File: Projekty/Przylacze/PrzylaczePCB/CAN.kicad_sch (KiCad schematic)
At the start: 49 parts, among them SW1 SW_SPDT, SW2 SW_SPDT, SW3 SW_SPDT, SW4 SW_SPDT, SW5 SW_SPDT, SW6 SW_SPDT, SW7 SW_SPDT, SW8 SW_SPDT, U1 MCP2515-xSO, U2 TJA1055T_3_C,518, U3 MCP2561-E-P, Y1 20MHz

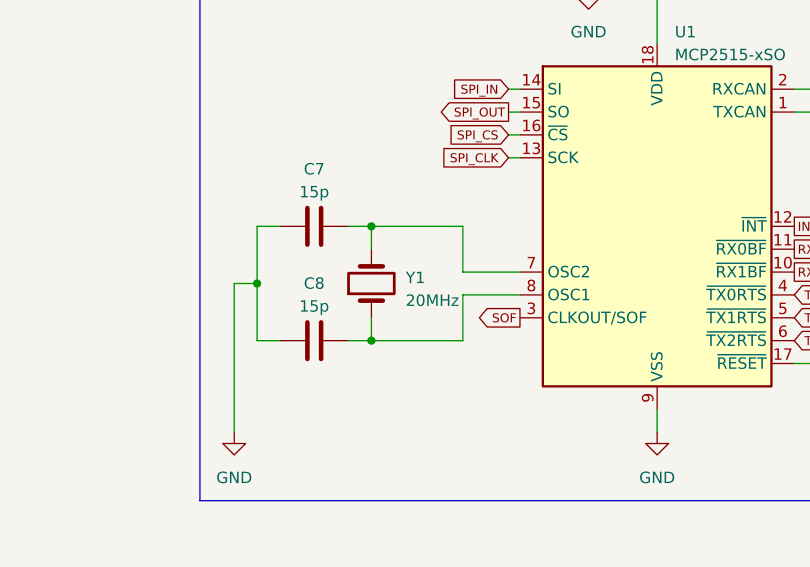
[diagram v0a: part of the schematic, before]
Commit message: Przyłącze - projekt PCB v0.2
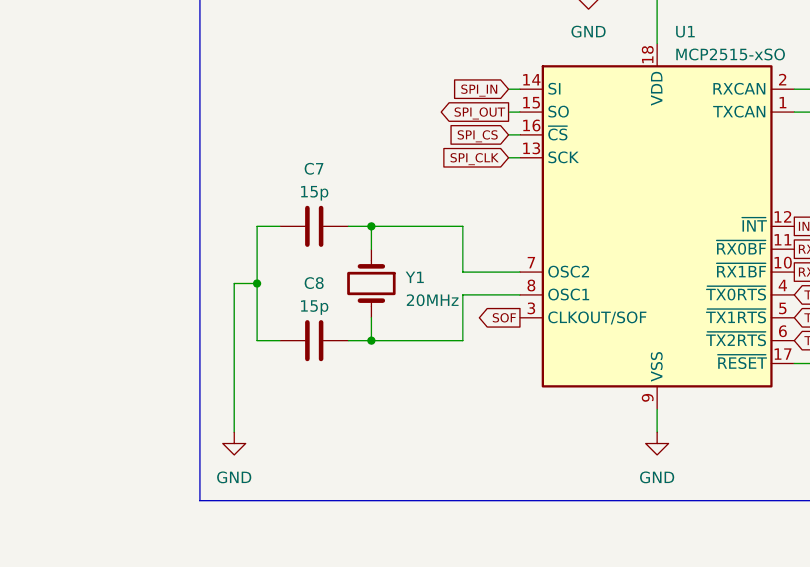
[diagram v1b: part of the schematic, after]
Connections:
- net at C7.2, U1.7 (OSC2): now also Y1.1; no longer Y1.2
- net at C8.2, U1.8 (OSC1): now also Y1.2; no longer Y1.1
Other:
- moved on the sheet: Y1

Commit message: Przyłącze - projekt PCB v1.1
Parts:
- D3, D4, D5: footprint 1_WLASNA_Library:2PAD_WIRE -> Connector_PinHeader_2.54mm:PinHeader_1x02_P2.54mm_Vertical
- H1: footprint 1_WLASNA_Library:4Pin_COMMON_MODE_CHOKE_B82787C0104H002 -> PrzylaczeFootprintLibrary:4Pin_COMMON_MODE_CHOKE_B82787C0104H002
- SW1, SW2, SW3, SW4, SW5, SW6, SW7, SW8: footprint 1_WLASNA_Library:3PAD_WIRE_SWITCH -> Connector_PinHeader_2.54mm:PinHeader_1x03_P2.54mm_Vertical
